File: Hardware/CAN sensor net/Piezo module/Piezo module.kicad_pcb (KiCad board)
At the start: 4 copper layers, 38.3 x 25.1 mm, 90 parts, among them J1 532610671, J2 532610671, J3 USB_B_Micro, J4 530470310, J5 532610271, SW1 SW_Push, SW2 SW_SPDT, U1 SN65HVD230, U2 STM32F103C8Tx, U3 W25Q32FVSSIG, U4 L78L05_SOT89, U5 LD3985M33R_SOT23, U6 L79L05_SOT89, U7 USBLC6-2SC6, U8 TL072, U9 ADS1120-PW, Y1 16MHz

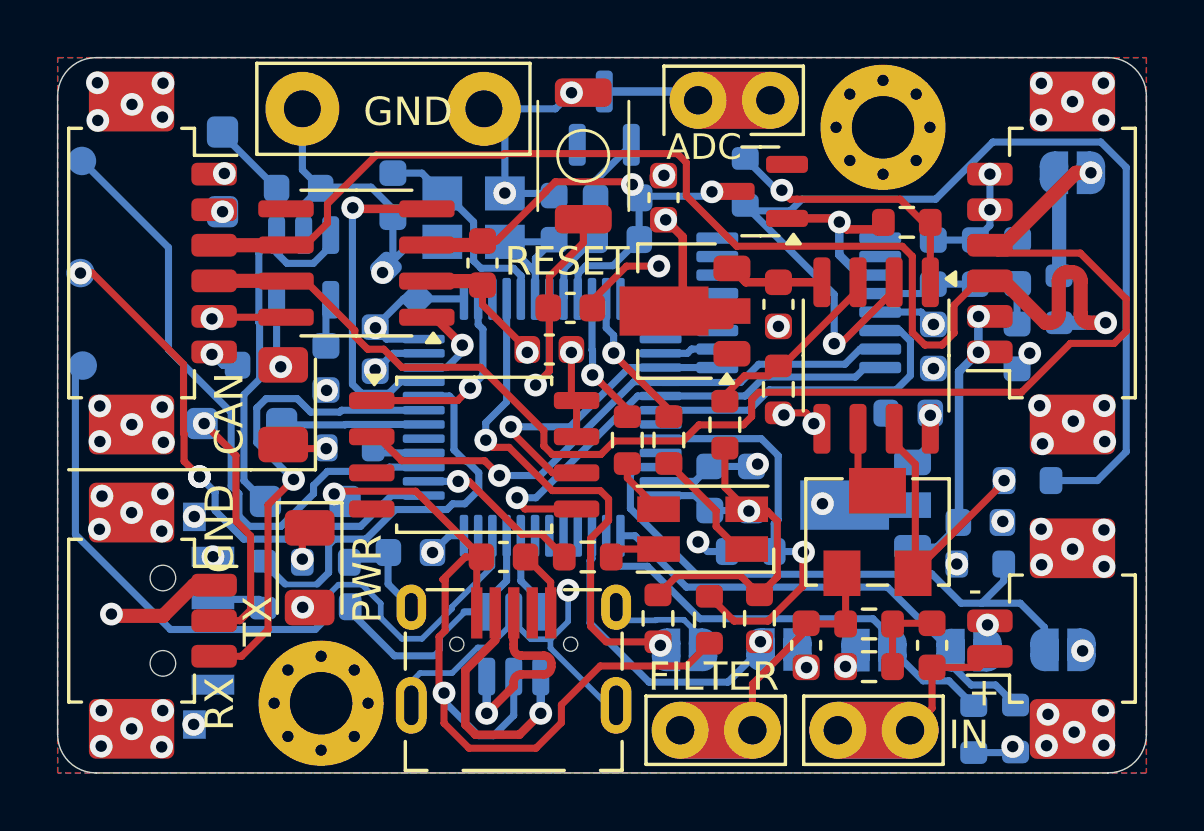
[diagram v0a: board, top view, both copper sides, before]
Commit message: Finished piezo board
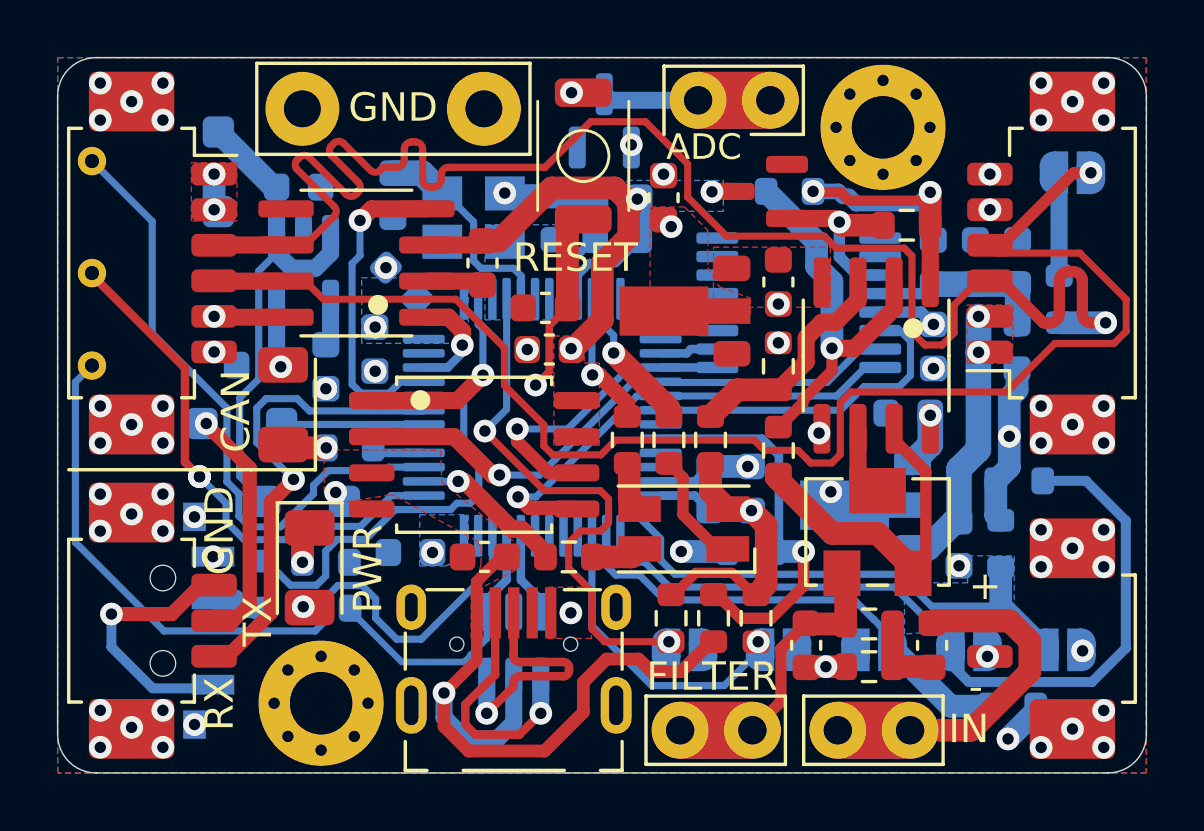
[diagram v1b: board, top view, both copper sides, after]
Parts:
- R20: moved to F.Cu
- TP5, TP6, TP7: footprint TestPoint:TestPoint_Pad_D1.0mm -> TestPoint:TestPoint_THTPad_D1.0mm_Drill0.5mm
- moved R20 8.82 mm to (158.0, 102.2), turned to 90 degrees
- moved R11 8.70 mm to (166.5, 103.3), turned to 180 degrees
- moved R21 1.59 mm to (158.4, 93.1), turned to 0 degrees
- moved R10 1.58 mm to (166.2, 111.2), turned to 0 degrees
- moved C17 1.06 mm to (164.3, 105.5), turned to -90 degrees
- moved R12 1.01 mm to (165.8, 105.5), turned to 90 degrees
- moved C1 0.88 mm to (149.8, 97.2), turned to 0 degrees
- moved R17 0.81 mm to (158.0, 99.2), turned to 90 degrees
- moved C14 0.79 mm to (158.0, 96.3)
- moved R16 0.74 mm to (155.6, 101.8)
- moved D2 0.67 mm to (154.7, 105.0)
- moved C20 0.66 mm to (147.7, 105.9), turned to 180 degrees
- moved R4 0.66 mm to (150.6, 105.9)
- moved R8 0.46 mm to (154.2, 108.1)
- moved TP6 0.40 mm to (133.9, 96.0)
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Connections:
- C25 pad 1: Net-(J5-Pin_1) -> Net-(J5-Pin_2)
- J5 pad 1: Net-(J5-Pin_1) -> GND
- J5 pad 2: GND -> Net-(J5-Pin_2)
- TP2 pad 1: Net-(J5-Pin_1) -> Net-(J5-Pin_2)
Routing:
- net GND: track 84.1 -> 37.7 mm, vias 26 -> 25
- net VDD_7V0: track 47.0 -> 15.8 mm
- net Net-(U8A--): track 37.3 -> 13.7 mm
- net Net-(J5-Pin_2): track 0.00 -> 20.1 mm
- net Net-(J5-Pin_1): track 14.9 -> 0.00 mm
- net ADDR_1: track 16.6 -> 29.1 mm
- net VDD_3V3: track 48.4 -> 60.7 mm, vias 13 -> 12
- net CAN_-: track 44.8 -> 55.2 mm
- net VDD_5V_USB: track 32.9 -> 25.3 mm
- net RCC_OSC_OUT: track 6.57 -> 0.00 mm
- net Net-(D6-A): track 25.3 -> 30.5 mm
- net VDD_-5V0: track 3.36 -> 0.00 mm
- net Net-(R18-Pad1): track 9.54 -> 12.8 mm, vias 1 -> 2
- net Net-(R20-Pad1): track 9.96 -> 12.2 mm, vias 1 -> 0
- net CAN_+: track 48.5 -> 50.6 mm
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- added copper zone on B.Cu, net ADDR_0
- added copper zone on B.Cu, net RCC_OSC_OUT
- added copper zone on F.Cu, net VDD_-5V0
- added copper zone on B.Cu, net VDD_3V3
- added copper zone on F.Cu, net VDD_3V3
- added copper zone on F.Cu, net VDD_5V_USB
- added copper zone on F.Cu, net VDD_7V0
- added copper zone on In1.Cu, net VDD_7V0
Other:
- board text added: "добавить MP у остальных плат 4 -> 0 или 0 -> 4 piezo + can out"
- board text removed: "CAN_OUT"
- board text removed: "PIEZO"
- board text removed: "концепт: перетрассировать полностью проверить существующие подписи (+ подписи коннекторов и терминатора?) проверить заливки добавить MP у остальных плат"
